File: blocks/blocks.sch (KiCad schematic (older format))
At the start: 0 parts

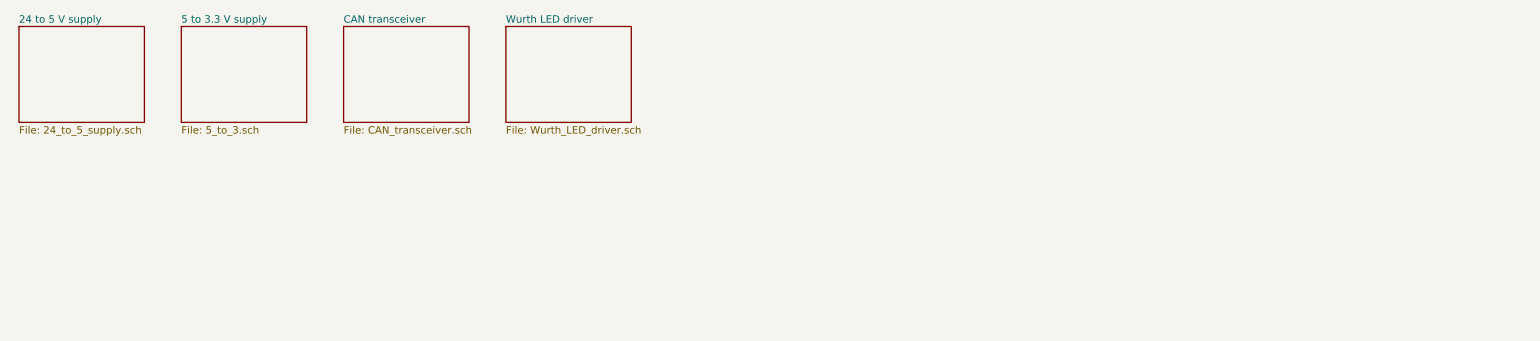
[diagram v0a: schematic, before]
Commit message: added multiple schematics
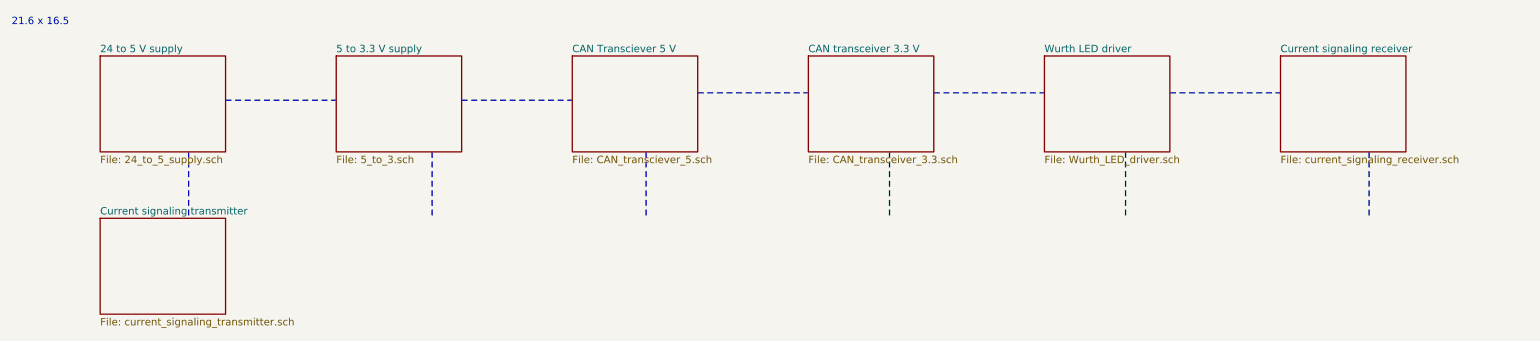
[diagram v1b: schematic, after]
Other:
- note added: "21.6 x 16.5"
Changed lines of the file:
@@
 EESchema Schematic File Version 4
+LIBS:blocks-cache
 EELAYER 29 0
 EELAYER END
 $Descr A4 11693 8268
 encoding utf-8
-Sheet 1 4
-Title ""
-Date ""
-Rev ""
-Comp ""
-Comment1 ""
-Comment2 ""
-Comment3 ""
-Comment4 ""
+Sheet 1 8
+Title "Schematic Blocks"
+Date "2019-12-05"
+Rev "1.0"
+Comp "KTH Formula Student"
+Comment1 " - "
+Comment2 "Jordi Altayó"
+Comment3 "jordiag@kth.se"
+Comment4 "Top page"
 $EndDescr
 $Sheet
-S 650  650  850  650
+S 1200 850  850  650
 U 5DE839B2
 F0 "24 to 5 V supply" 50
@@
 $EndSheet
 $Sheet
-S 1750 650  850  650
+S 9200 850  850  650
+U 5DE842DA
+F0 "Current signaling receiver" 50
+F1 "current_signaling_receiver.sch" 50
+$EndSheet
+$Sheet
+S 7600 850  850  650
+U 5DE83B88
+F0 "Wurth LED driver" 50
+F1 "Wurth_LED_driver.sch" 50
+$EndSheet
+$Sheet
+S 6000 850  850  650
+U 5DE83A8B
+F0 "CAN transceiver 3.3 V" 50
+F1 "CAN_transceiver_3.3.sch" 50
+$EndSheet
+$Sheet
+S 2800 850  850  650
 U 5DE839FC
 F0 "5 to 3.3 V supply" 50
@@
 $EndSheet
 $Sheet
-S 2850 650  850  650
-U 5DE83A8B
-F0 "CAN transceiver" 50
-F1 "CAN_transceiver.sch" 50
+S 1200 1950 850  650
+U 5DE84438
+F0 "Current signaling transmitter" 50
+F1 "current_signaling_transmitter.sch" 50
 $EndSheet
+Wire Notes Line
+	3650 1150 4400 1150
+Wire Notes Line
+	2050 1150 2800 1150
+Wire Notes Line
+	5250 1100 6000 1100
+Wire Notes Line
+	6850 1100 7600 1100
+Wire Notes Line
+	8450 1100 9200 1100
+Wire Notes Line
+	1800 1500 1800 1950
+Wire Notes Line
+	3450 1500 3450 1950
+Wire Notes Line
+	4900 1500 4900 1950
+Wire Notes Line
+	6550 1500 6550 1950
+Wire Notes Line
+	8150 1500 8150 1950
+Wire Notes Line
+	9800 1500 9800 1950
+Text Notes 600  650  0    50   ~ 0
+21.6 x 16.5
 $Sheet
-S 3950 650  850  650
-U 5DE83B88
-F0 "Wurth LED driver" 50
-F1 "Wurth_LED_driver.sch" 50
+S 4400 850  850  650
+U 5DEB58F1
+F0 "CAN Transciever 5 V" 50
+F1 "CAN_transciever_5.sch" 50
 $EndSheet
 $EndSCHEMATC
